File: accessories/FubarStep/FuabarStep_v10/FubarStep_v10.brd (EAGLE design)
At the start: 71.1 x 85.7 mm, 10 parts, among them IC1 7805, X1 DC21MMX

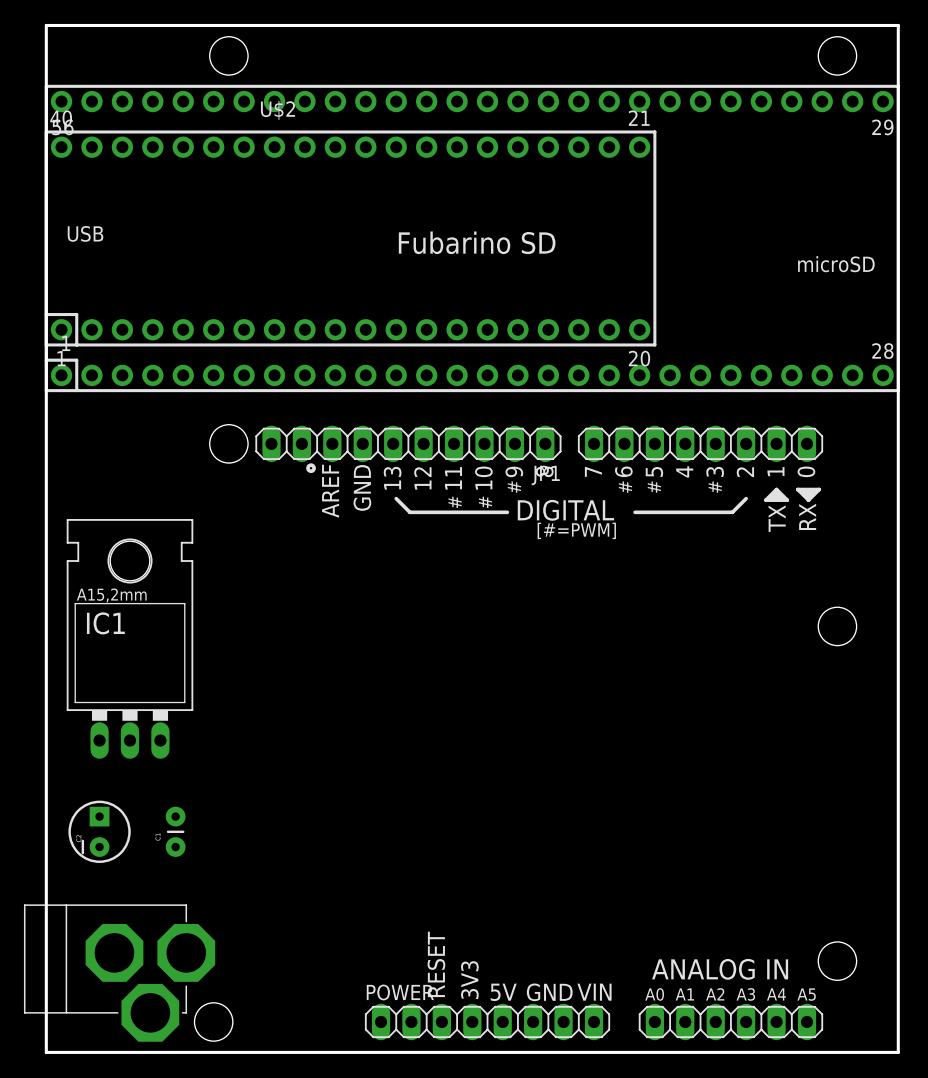
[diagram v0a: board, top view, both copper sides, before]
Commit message: More work.
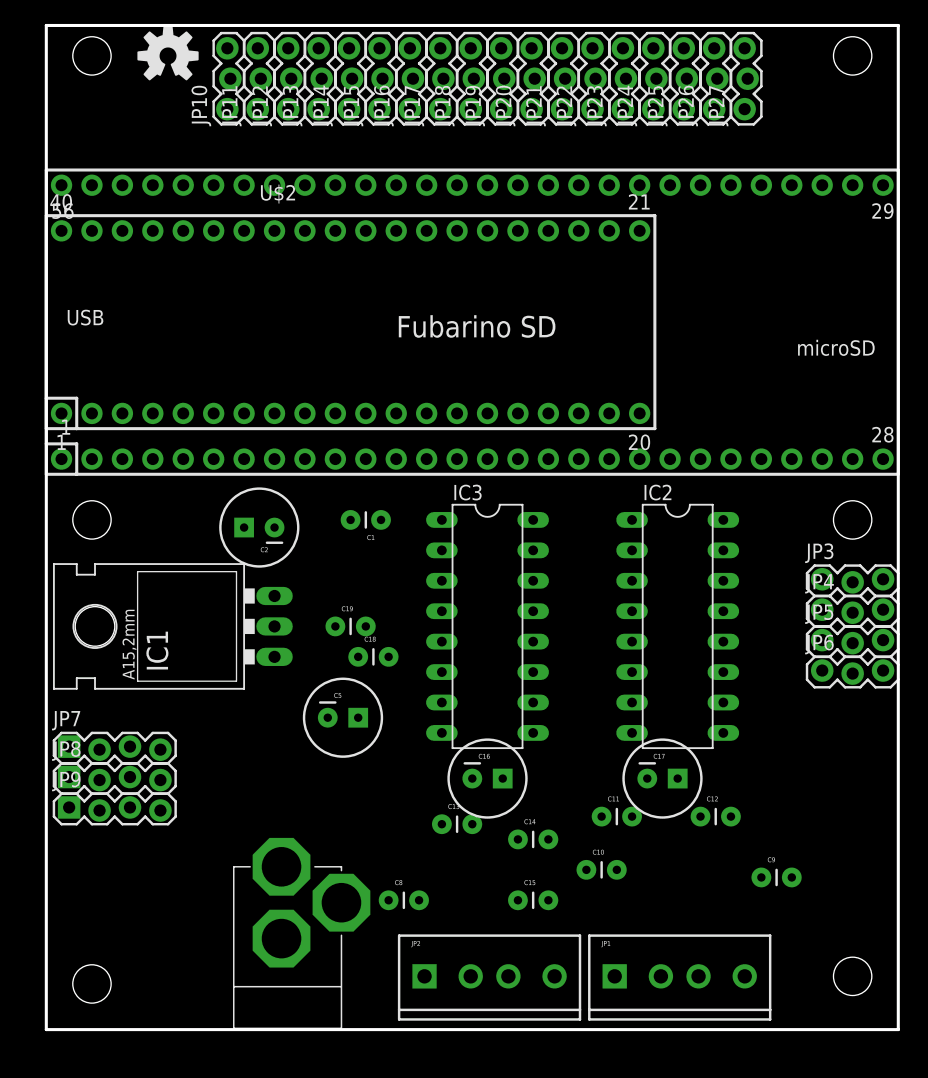
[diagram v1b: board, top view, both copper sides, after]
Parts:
- removed AD: (no value), pinhead:1X06
- removed IOL, POWER: (no value), pinhead:1X08
- added C10, C11, C12, C13, C14, C15, C18, C19, C8, C9: .1uF, SparkFun-Capacitors:CAP-PTH-SMALL
- added C16, C17, C5: 100uF, SparkFun-Capacitors:CPOL-RADIAL-100UF-25V
- added IC2, IC3: SN754410NE, texas:DIL16
- added JP10, JP11, JP12, JP13, JP14, JP15, JP16, JP17, JP18, JP19, JP20, JP21, JP22, JP23, JP24, JP25, JP26, JP27, JP3, JP4, JP5, JP6: (no value), SparkFun-Connectors:1X03_LOCK
- added JP2: (no value), SparkFun-Connectors:SCREWTERMINAL-3.5MM-4_LOCK
- added JP7, JP8, JP9: (no value), SparkFun-Connectors:1X04_LOCK
- added LOGO1: OSHW-LOGOM, SparkFun-Aesthetics:OSHW-LOGO-M
- C2: value 10uF -> 100uF; device SparkFun-Capacitors:CPOL-RADIAL-10UF-25V -> SparkFun-Capacitors:CPOL-RADIAL-100UF-25V
- IC1: value 7805 -> OKI-78SR-5/1.5-W36H-C
- JP1: device pinhead:1X10 -> SparkFun-Connectors:SCREWTERMINAL-3.5MM-4_LOCK
- moved JP1 47.7 mm to (47.6, 6.35), turned to 0 degrees
- moved C1 32.2 mm to (27.9, 44.5), turned to 180 degrees
- moved C2 28.7 mm to (17.8, 43.8), turned to 180 degrees
- moved X1 14.2 mm to (19.6, 9.14), turned to 180 degrees
- moved IC1 10.0 mm to (15.2, 35.6), turned to 90 degrees
- moved U$1 6.98 mm to (35.6, 61.0)
- moved U$2 6.98 mm to (25.4, 61.0)
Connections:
- removed net AD0: AD.1
- removed net AD1: AD.2
- removed net AD2: AD.3
- removed net AD3: AD.4
- removed net AD4: AD.5
- removed net AD4/SDA: JP1.9
- removed net AD5: AD.6
- removed net AD5/SCL: JP1.10
- removed net AREF: JP1.8
- removed net IO0: IOL.1
- removed net IO1: IOL.2
- removed net IO2: IOL.3
- removed net IO3: IOL.4
- removed net IO4: IOL.5
- removed net IO5: IOL.6
- removed net IO6: IOL.7
- removed net IO7: IOL.8
- removed net IO8: JP1.1
- removed net IO9: JP1.2
- removed net MISO: JP1.5
- removed net MOSI: JP1.4
- removed net SCK: JP1.6
- removed net SS: JP1.3
- new net M1A1: IC2.2
- new net M1A2: IC2.7
- new net M1A3: IC2.10
- new net M1A4: IC2.15
- new net M1EN12: IC2.1, U$1.11
- new net M1EN34: IC2.9, U$1.12
- new net M1O1: C10.2, IC2.3, JP1.1
- new net M1O2: C11.2, IC2.6, JP1.2
- new net M1O3: C12.1, IC2.11, JP1.3
- new net M1O4: C9.1, IC2.14, JP1.4
- new net M2A1: IC3.2
- new net M2A2: IC3.7
- new net M2A3: IC3.10
- new net M2A4: IC3.15
- new net M2EN12: IC3.1, U$1.13
- new net M2EN34: IC3.9, U$1.14
- new net M2O1: C8.2, IC3.3, JP2.1
- new net M2O2: C13.2, IC3.6, JP2.2
- new net M2O3: C15.1, IC3.11, JP2.3
- new net M2O4: C14.1, IC3.14, JP2.4
- new net N$12: JP8.1
- new net N$2: JP18.1
- new net N$29: JP9.1
- new net N$3: JP19.1
- new net N$67: JP9.2
- new net N$68: JP9.3
- new net N$69: JP23.1
- new net N$87: JP22.1
- new net N$88: JP17.1
- new net N$89: JP16.1
- new net N$90: JP15.1
- new net N$91: JP14.1
- new net N$92: JP10.1
- new net N$93: JP11.1
- new net N$94: JP12.1
- new net N$95: JP13.1
- new net N$96: JP24.1
- new net N$97: JP25.1
- new net RX: JP7.3, U$1.52
- new net SERVO1: JP6.1
- new net SERVO2: JP3.1
- new net SERVO3: JP4.1
- new net SERVO4: JP5.1
- new net TX: JP7.2, U$1.53
- net +3V3: no longer POWER.4
- net +5V: now also C18.1, C19.1, C5.1, IC2.16, IC3.16, JP10.2, JP11.2, JP12.2, JP13.2, JP14.2, JP15.2, JP16.2, JP17.2, JP18.2, JP19.2, JP20.2, JP21.2, JP22.2, JP23.2, JP24.2, JP25.2, JP26.2, JP27.2, JP3.2, JP4.2, JP5.2, JP6.2, JP7.1, U$1.56, U$2.40; no longer POWER.2, POWER.5, U$1.1, U$2.1
- net GND: now also C10.1, C11.1, C12.2, C13.1, C14.2, C15.2, C16.2, C17.2, C18.2, C19.2, C5.2, C8.1, C9.2, IC2.12, IC2.13, IC2.4, IC2.5, IC3.12, IC3.13, IC3.4, IC3.5, JP10.3, JP11.3, JP12.3, JP13.3, JP14.3, JP15.3, JP16.3, JP17.3, JP18.3, JP19.3, JP20.3, JP21.3, JP22.3, JP23.3, JP24.3, JP25.3, JP26.3, JP27.3, JP3.3, JP4.3, JP5.3, JP6.3, JP7.4, JP8.4, JP9.4; no longer JP1.7, POWER.6, POWER.7
- net N$11: now also JP20.1; no longer U$1.11
- net N$13: now also JP8.2; no longer U$1.12
- net N$14: now also JP8.3; no longer U$1.13
- net N$15: now also JP21.1; no longer U$1.14
- net N$33: now also JP26.1; no longer U$1.53
- net N$34: now also JP27.1; no longer U$1.52
- net RESET: no longer POWER.3
- net VIN: now also C16.1, C17.1, IC2.8, IC3.8; no longer POWER.8, U$1.56, U$2.40
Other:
- board size 71.1 x 85.7 mm -> 71.1 x 83.8 mm
- board text removed: "#"
- board text removed: "0"
- board text removed: "1"
- board text removed: "10"
- board text removed: "11"
- board text removed: "12"
- board text removed: "13"
- board text removed: "2"
- board text removed: "3"
- board text removed: "3V3"
- board text removed: "4"
- board text removed: "5"
- board text removed: "5V"
- board text removed: "6"
- board text removed: "7"
- board text removed: "8"
- board text removed: "9"
- board text removed: "A0"
- board text removed: "A1"
- board text removed: "A2"
- board text removed: "A3"
- board text removed: "A4"
- board text removed: "A5"
- board text removed: "ANALOG IN"
- board text removed: "AREF"
- board text removed: "DIGITAL"
- board text removed: "GND"
- board text removed: "RESET"
- board text removed: "RX"
- board text removed: "TX"
- board text removed: "VIN"
- board text removed: "[#=PWM]"
